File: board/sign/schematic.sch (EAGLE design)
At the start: 37 parts, among them IC1 STM32F207ZGT, IC3 LM3940, J1 DCJ0202, X2 22-23-2041

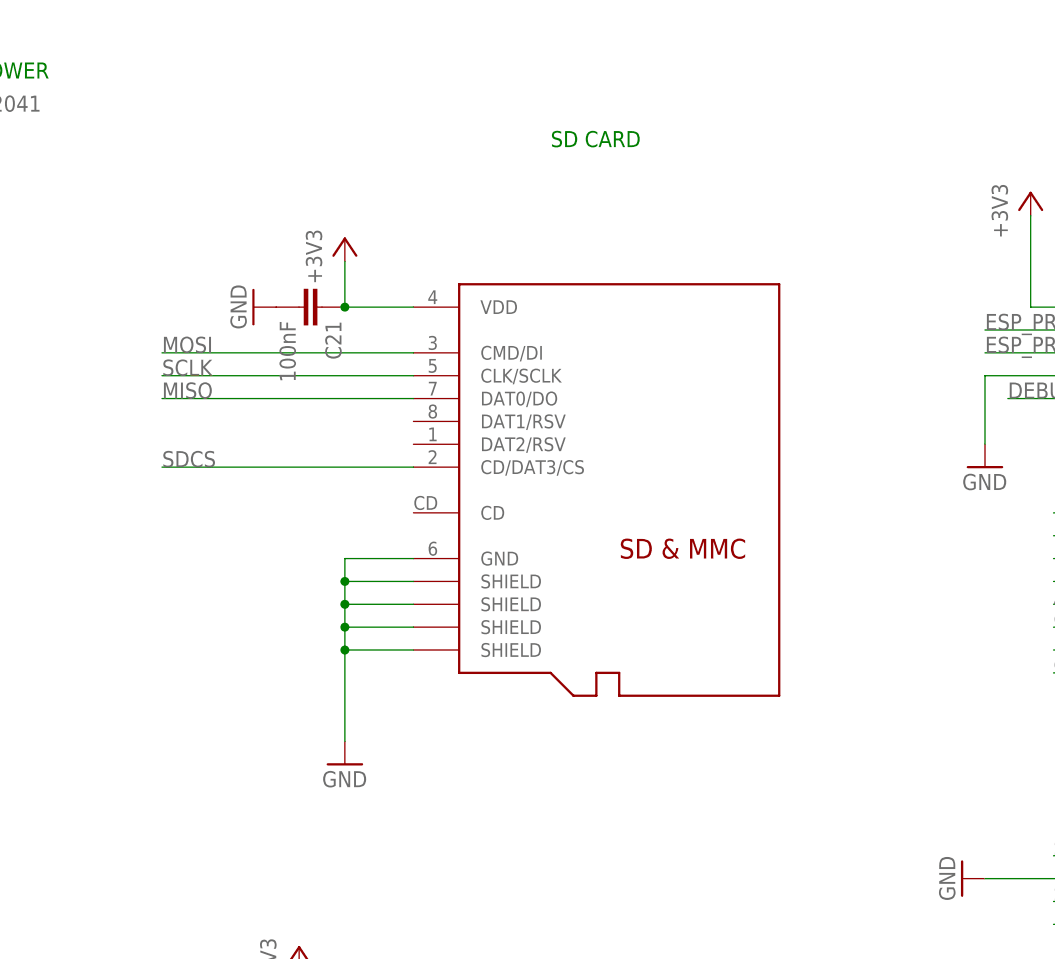
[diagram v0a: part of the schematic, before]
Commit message: Fix SD
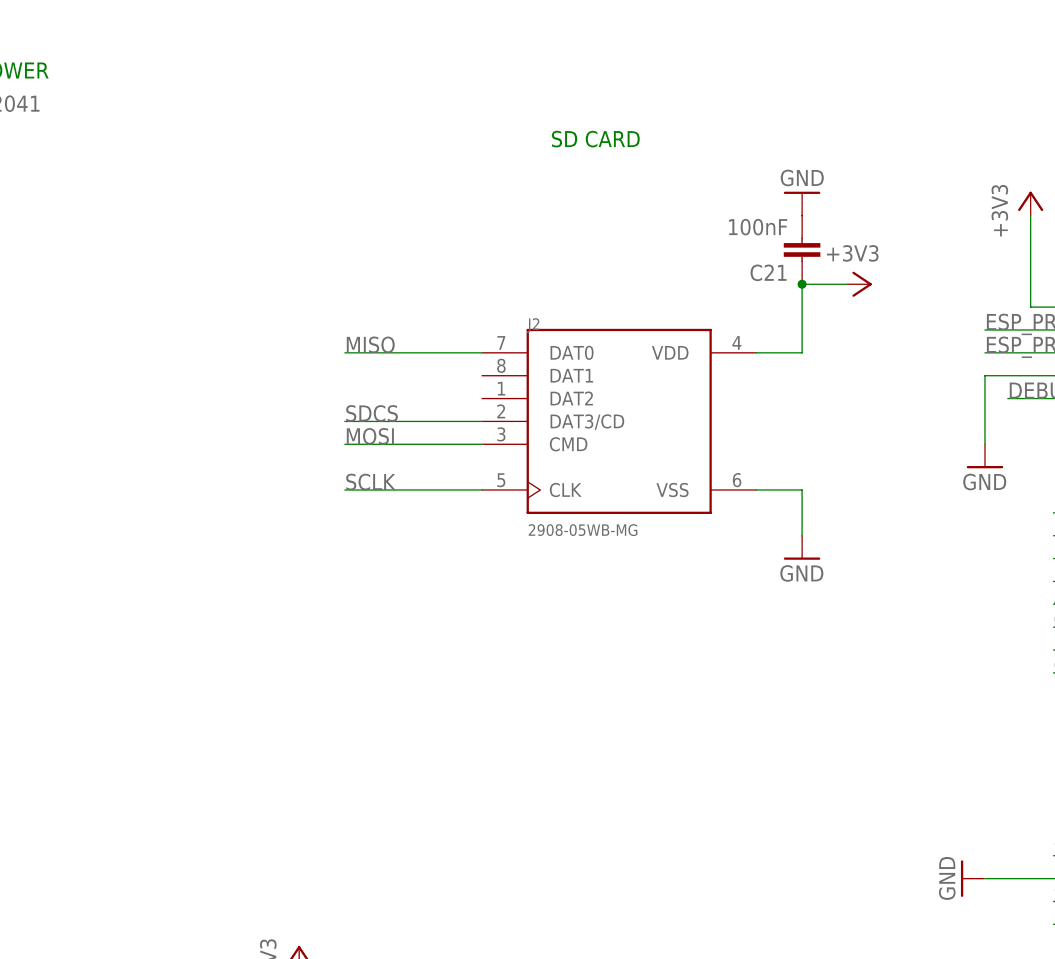
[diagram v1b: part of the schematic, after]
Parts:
- removed U$1: MICROSD, micro-sd:MICROSD
- added J2: 2908-05WB-MG, 2908-05WB-MG:2908-05WB-MG
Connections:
- net +3V3: now also J2.VDD; no longer U$1.VDD
- net GND: now also J2.VSS; no longer U$1.GND, U$1.SHIELD@1, U$1.SHIELD@2, U$1.SHIELD@3, U$1.SHIELD@4
- net MISO: now also J2.DAT0; no longer U$1.DAT0/DO
- net MOSI: now also J2.CMD; no longer U$1.CMD/DI
- net SCLK: now also J2.CLK; no longer U$1.CLK/SCLK
- net SDCS: now also J2.DAT3/CD; no longer U$1.CD/DAT3/CS
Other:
- moved on the sheet: C21
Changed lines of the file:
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@@
 <part name="R2" library="rcl" library_urn="urn:adsk.eagle:library:334" deviceset="R-US_" device="0204/7" package3d_urn="urn:adsk.eagle:package:23498/1" value="12k"/>
 <part name="GND11" library="supply1" library_urn="urn:adsk.eagle:library:371" deviceset="GND" device=""/>
-<part name="U$1" library="micro-sd" deviceset="MICROSD" device=""/>
 <part name="+3V5" library="supply1" library_urn="urn:adsk.eagle:library:371" deviceset="+3V3" device=""/>
-<part name="GND12" library="supply1" library_urn="urn:adsk.eagle:library:371" deviceset="GND" device=""/>
 <part name="C21" library="rcl" library_urn="urn:adsk.eagle:library:334" deviceset="C-EU" device="025-025X050" package3d_urn="urn:adsk.eagle:package:23629/2" value="100nF"/>
 <part name="GND13" library="supply1" library_urn="urn:adsk.eagle:library:371" deviceset="GND" device=""/>
@@
 <part name="+3V2" library="supply1" library_urn="urn:adsk.eagle:library:371" deviceset="+3V3" device=""/>
 <part name="+3V11" library="supply1" library_urn="urn:adsk.eagle:library:371" deviceset="+3V3" device=""/>
+<part name="J2" library="2908-05WB-MG" deviceset="2908-05WB-MG" device=""/>
+<part name="GND20" library="supply1" library_urn="urn:adsk.eagle:library:371" deviceset="GND" device=""/>
 </parts>
 <sheets>
@@
 <attribute name="VALUE" x="86.36" y="15.24" size="1.778" layer="96"/>
 </instance>
-<instance part="U$1" gate="G$1" x="236.22" y="88.9" smashed="yes"/>
-<instance part="+3V5" gate="G$1" x="208.28" y="114.3" smashed="yes">
-<attribute name="VALUE" x="205.74" y="109.22" size="1.778" layer="96" rot="R90"/>
-</instance>
-<instance part="GND12" gate="1" x="208.28" y="55.88" smashed="yes">
-<attribute name="VALUE" x="205.74" y="53.34" size="1.778" layer="96"/>
-</instance>
-<instance part="C21" gate="G$1" x="205.74" y="106.68" smashed="yes" rot="R270">
-<attribute name="NAME" x="206.121" y="105.156" size="1.778" layer="95" rot="R270"/>
-<attribute name="VALUE" x="201.041" y="105.156" size="1.778" layer="96" rot="R270"/>
-</instance>
-<instance part="GND13" gate="1" x="198.12" y="106.68" smashed="yes" rot="R270">
-<attribute name="VALUE" x="195.58" y="109.22" size="1.778" layer="96" rot="R270"/>
+<instance part="+3V5" gate="G$1" x="266.7" y="109.22" smashed="yes" rot="R270">
+<attribute name="VALUE" x="261.62" y="111.76" size="1.778" layer="96"/>
+</instance>
+<instance part="C21" gate="G$1" x="259.08" y="111.76" smashed="yes" rot="R180">
+<attribute name="NAME" x="257.556" y="111.379" size="1.778" layer="95" rot="R180"/>
+<attribute name="VALUE" x="257.556" y="116.459" size="1.778" layer="96" rot="R180"/>
+</instance>
+<instance part="GND13" gate="1" x="259.08" y="119.38" smashed="yes" rot="R180">
+<attribute name="VALUE" x="261.62" y="121.92" size="1.778" layer="96" rot="R180"/>
 </instance>
 <instance part="X2" gate="-1" x="162.56" y="127" smashed="yes">
@@
 <instance part="+3V11" gate="G$1" x="289.56" y="215.9" smashed="yes">
 <attribute name="VALUE" x="287.02" y="210.82" size="1.778" layer="96" rot="R90"/>
+</instance>
+<instance part="J2" gate="G$1" x="238.76" y="93.98" smashed="yes">
+<attribute name="NAME" x="228.5841" y="104.1559" size="1.271990625" layer="95"/>
+<attribute name="VALUE" x="228.5925" y="81.2706" size="1.270940625" layer="96"/>
+</instance>
+<instance part="GND20" gate="1" x="259.08" y="78.74" smashed="yes">
+<attribute name="VALUE" x="256.54" y="76.2" size="1.778" layer="96"/>
 </instance>
 </instances>
@@
 </segment>
 <segment>
-<pinref part="GND12" gate="1" pin="GND"/>
-<pinref part="U$1" gate="G$1" pin="SHIELD@4"/>
-<wire x1="208.28" y1="58.42" x2="208.28" y2="68.58" width="0.1524" layer="91"/>
-<wire x1="208.28" y1="68.58" x2="215.9" y2="68.58" width="0.1524" layer="91"/>
-<pinref part="U$1" gate="G$1" pin="SHIELD@2"/>
-<wire x1="215.9" y1="73.66" x2="208.28" y2="73.66" width="0.1524" layer="91"/>
-<wire x1="208.28" y1="73.66" x2="208.28" y2="71.12" width="0.1524" layer="91"/>
-<junction x="208.28" y="68.58"/>
-<pinref part="U$1" gate="G$1" pin="SHIELD@3"/>
-<wire x1="208.28" y1="71.12" x2="208.28" y2="68.58" width="0.1524" layer="91"/>
-<wire x1="208.28" y1="71.12" x2="215.9" y2="71.12" width="0.1524" layer="91"/>
-<junction x="208.28" y="71.12"/>
-<pinref part="U$1" gate="G$1" pin="SHIELD@1"/>
-<wire x1="215.9" y1="76.2" x2="208.28" y2="76.2" width="0.1524" layer="91"/>
-<wire x1="208.28" y1="76.2" x2="208.28" y2="73.66" width="0.1524" layer="91"/>
-<junction x="208.28" y="73.66"/>
-<pinref part="U$1" gate="G$1" pin="GND"/>
-<wire x1="215.9" y1="78.74" x2="208.28" y2="78.74" width="0.1524" layer="91"/>
-<wire x1="208.28" y1="78.74" x2="208.28" y2="76.2" width="0.1524" layer="91"/>
-<junction x="208.28" y="76.2"/>
-</segment>
-<segment>
 <pinref part="C21" gate="G$1" pin="2"/>
 <pinref part="GND13" gate="1" pin="GND"/>
@@
 <pinref part="GND2" gate="1" pin="GND"/>
 <junction x="20.32" y="119.38"/>
+</segment>
+<segment>
+<pinref part="GND20" gate="1" pin="GND"/>
+<wire x1="259.08" y1="81.28" x2="259.08" y2="86.36" width="0.1524" layer="91"/>
+<pinref part="J2" gate="G$1" pin="VSS"/>
+<wire x1="259.08" y1="86.36" x2="254" y2="86.36" width="0.1524" layer="91"/>
 </segment>
 </net>
@@
 <segment>
 <pinref part="+3V5" gate="G$1" pin="+3V3"/>
-<pinref part="U$1" gate="G$1" pin="VDD"/>
-<wire x1="208.28" y1="111.76" x2="208.28" y2="106.68" width="0.1524" layer="91"/>
-<wire x1="208.28" y1="106.68" x2="215.9" y2="106.68" width="0.1524" layer="91"/>
+<wire x1="264.16" y1="109.22" x2="259.08" y2="109.22" width="0.1524" layer="91"/>
+<wire x1="259.08" y1="109.22" x2="259.08" y2="101.6" width="0.1524" layer="91"/>
 <pinref part="C21" gate="G$1" pin="1"/>
-<junction x="208.28" y="106.68"/>
+<junction x="259.08" y="109.22"/>
+<pinref part="J2" gate="G$1" pin="VDD"/>
+<wire x1="259.08" y1="101.6" x2="254" y2="101.6" width="0.1524" layer="91"/>
 </segment>
 <segment>
@@
 <net name="SCLK" class="0">
 <segment>
-<pinref part="U$1" gate="G$1" pin="CLK/SCLK"/>
-<wire x1="215.9" y1="99.06" x2="187.96" y2="99.06" width="0.1524" layer="91"/>
-<label x="187.96" y="99.06" size="1.778" layer="95"/>
-</segment>
-<segment>
 <pinref part="IC2" gate="G$1" pin="GPIO14"/>
 <wire x1="27.94" y1="35.56" x2="17.78" y2="35.56" width="0.1524" layer="91"/>
 <label x="17.78" y="35.56" size="1.778" layer="95"/>
 </segment>
+<segment>
+<pinref part="J2" gate="G$1" pin="CLK"/>
+<wire x1="223.52" y1="86.36" x2="208.28" y2="86.36" width="0.1524" layer="91"/>
+<label x="208.28" y="86.36" size="1.778" layer="95"/>
+</segment>
 </net>
 <net name="MOSI" class="0">
-<segment>
-<pinref part="U$1" gate="G$1" pin="CMD/DI"/>
-<wire x1="215.9" y1="101.6" x2="187.96" y2="101.6" width="0.1524" layer="91"/>
-<label x="187.96" y="101.6" size="1.778" layer="95"/>
-</segment>
 <segment>
 <pinref part="IC2" gate="G$1" pin="GPIO4"/>
@@
 <label x="68.58" y="48.26" size="1.778" layer="95" rot="R90"/>
 </segment>
+<segment>
+<pinref part="J2" gate="G$1" pin="CMD"/>
+<wire x1="223.52" y1="91.44" x2="208.28" y2="91.44" width="0.1524" layer="91"/>
+<label x="208.28" y="91.44" size="1.778" layer="95"/>
+</segment>
 </net>
 <net name="MISO" class="0">
-<segment>
-<pinref part="U$1" gate="G$1" pin="DAT0/DO"/>
-<wire x1="215.9" y1="96.52" x2="187.96" y2="96.52" width="0.1524" layer="91"/>
-<label x="187.96" y="96.52" size="1.778" layer="95"/>
-</segment>
 <segment>
 <pinref part="IC2" gate="G$1" pin="GPIO12"/>
@@
 <label x="10.16" y="33.02" size="1.778" layer="95"/>
 </segment>
+<segment>
+<pinref part="J2" gate="G$1" pin="DAT0"/>
+<wire x1="223.52" y1="101.6" x2="208.28" y2="101.6" width="0.1524" layer="91"/>
+<label x="208.28" y="101.6" size="1.778" layer="95"/>
+</segment>
 </net>
 <net name="SDCS" class="0">
-<segment>
-<pinref part="U$1" gate="G$1" pin="CD/DAT3/CS"/>
-<wire x1="215.9" y1="88.9" x2="187.96" y2="88.9" width="0.1524" layer="91"/>
-<label x="187.96" y="88.9" size="1.778" layer="95"/>
-</segment>
 <segment>
 <pinref part="IC2" gate="G$1" pin="GPIO5"/>
@@
 <label x="66.04" y="48.26" size="1.778" layer="95" rot="R90"/>
 </segment>
-</net>
+<segment>
+<pinref part="J2" gate="G$1" pin="DAT3/CD"/>
+<wire x1="223.52" y1="93.98" x2="208.28" y2="93.98" width="0.1524" layer="91"/>
+<label x="208.28" y="93.98" size="1.778" layer="95"/>
+</segment>
+</net>
